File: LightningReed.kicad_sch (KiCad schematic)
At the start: 175 parts, among them P1 Conn_WallPlug, Q1 NCE65T180D, Q10 DMZ6005E, Q11 2N7002K, Q12 NCEP15T14D, Q13 BSS123, Q2 2N7002, Q3 1N60G, Q4 2N7002, Q5 2N7002K, Q6 2N7002K, Q7 CMSA65R280Q, Q8 CMSA65R280Q, Q9 NCE0102, T1 Transformer_2P_2S, U1 UCC28056, U2 78L05S, U3 LMC7111, U4 UCC28780, U5 UCC27712, U6 LM317LCPK, U7 FODM8801A, U8 TL431DBZ, U9 UCC24612-1DBV

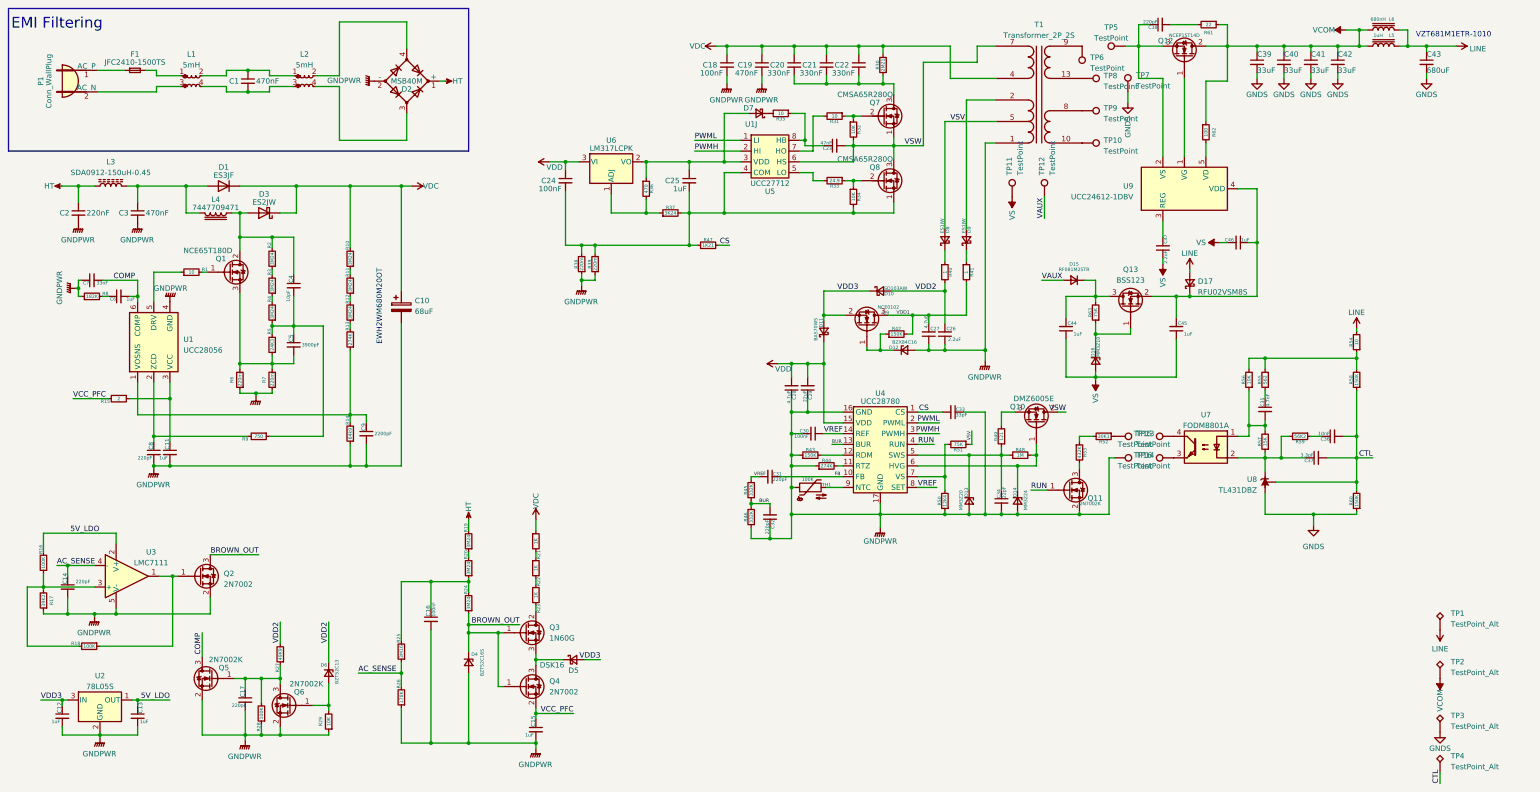
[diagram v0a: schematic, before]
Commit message: Controller 50%
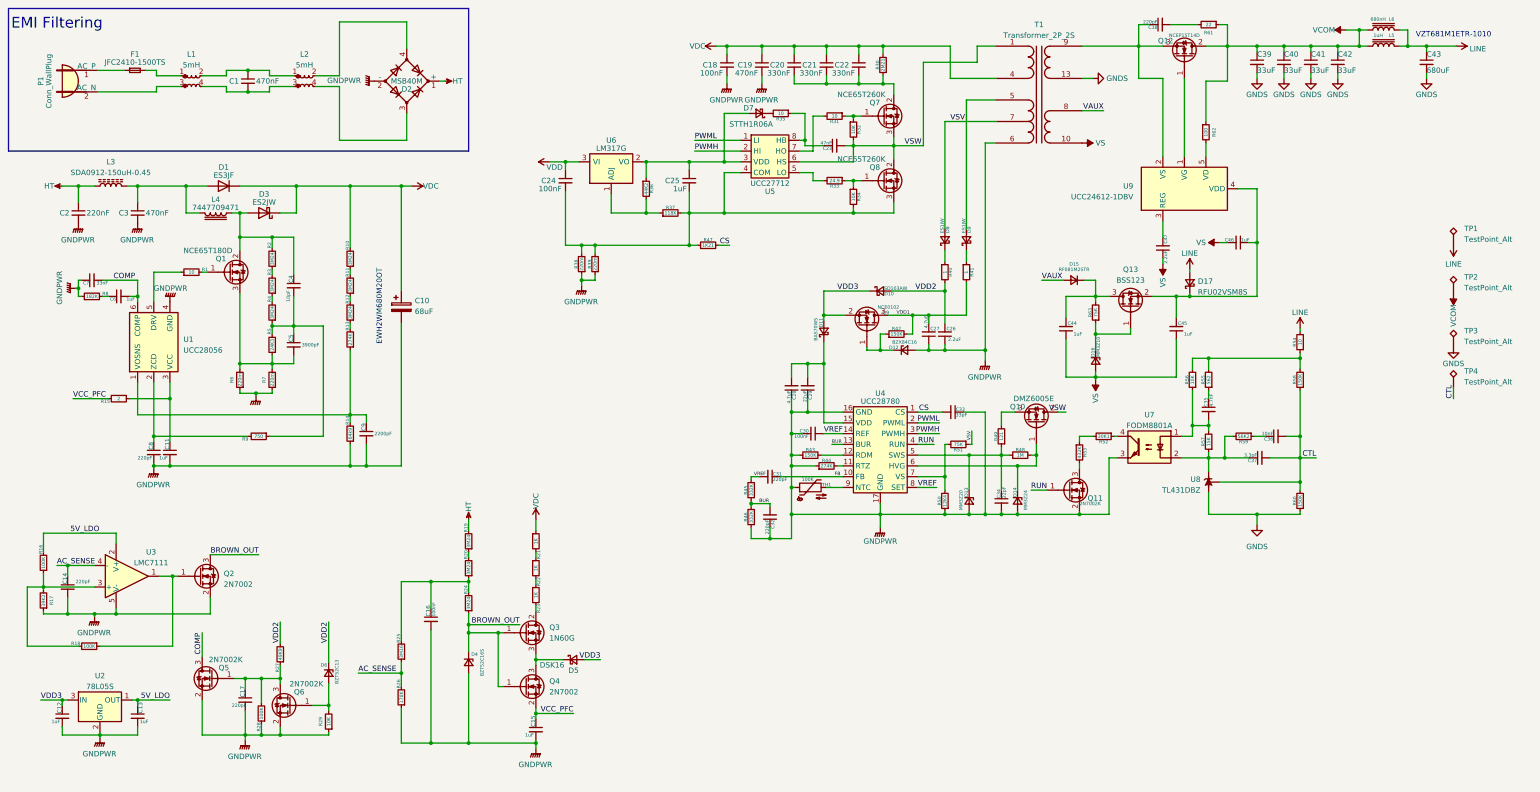
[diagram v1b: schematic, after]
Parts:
- removed Q7: CMSA65R280Q, Package_SON:VSONP-8-1EP_5x6_P1.27mm, symbol Device:Q_NMOS_SGD
- removed TP10, TP11, TP12, TP13, TP14, TP15, TP16, TP9: TestPoint, Connector_Wire:SolderWire-0.15sqmm_1x01_D0.5mm_OD1.5mm, symbol Connector:TestPoint
- removed TP5, TP6, TP7, TP8: TestPoint, Connector_Wire:SolderWire-1sqmm_1x01_D1.4mm_OD2.7mm, symbol Connector:TestPoint
- added Q7: NCE65T260K, Package_TO_SOT_SMD:TO-252-2, symbol Device:Q_NMOS_GDS
- D7: value U1J -> STTH1R06A; footprint Diode_SMD:D_SOD-123F -> Diode_SMD:D_SMA
- Q8: value CMSA65R280Q -> NCE65T260K; footprint Package_SON:VSONP-8-1EP_5x6_P1.27mm -> Package_TO_SOT_SMD:TO-252-2; symbol Device:Q_NMOS_SGD -> Device:Q_NMOS_GDS
- R36: value 470 -> 44K2
- R37: value 3K24 -> 118K
- TP1: footprint Connector_Wire:SolderWire-1sqmm_1x01_D1.4mm_OD2.7mm -> Connector_Wire:SolderWire-0.5sqmm_1x01_D0.9mm_OD2.1mm
- U2: footprint Package_TO_SOT_SMD:SOT-23 -> Package_TO_SOT_SMD:SOT-89-3
- U6: value LM317LCPK -> LM317G; footprint Package_TO_SOT_SMD:SOT-89-3 -> Package_TO_SOT_SMD:SOT-223-3_TabPin2; symbol Regulator_Linear:LM317L_SOT-89 -> Regulator_Linear:NCP1117-ADJ_SOT223
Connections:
- net GNDPWR: now also T1.6 (SD), U7.3; no longer T1.1 (SD)
- net GNDS: now also T1.13 (SB)
- net VAUX: now also T1.8 (SC)
- net VDD: no longer C28.2, C29.2, D11.1 (K), U4.15 (VDD)
- net VS: now also T1.10 (SD)
- net VSV: now also T1.7 (SD); no longer T1.5 (SD)
- net VSW: now also Q8.2 (D), T1.1 (AA), Q7.3 (S); no longer Q8.3 (D), T1.7 (AA)
- net at R31.1, R32.1: now also Q7.1 (G)
- net at C20.2, C21.2, C22.2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: now also Q7.2 (D)
- net at R33.1, R34.1: now also Q8.1 (G); no longer Q8.2 (G)
- net at C24.2, C25.2, R34.2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: now also Q8.3 (S); no longer Q8.1 (S)
- net at R52.1: now also U7.4
- net at C38.1, Q12.3 (S), U9.2 (VS): now also T1.9 (SA)
- net at D9.2 (A): now also T1.5 (SC); no longer T1.2 (SC)
- new net: C28.2, C29.2, D11.1 (K), U4.15 (VDD)
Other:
- moved on the sheet: C35, C36, C37, R54, R55, R56, R57, R58, R59, R60, TP1, TP2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
